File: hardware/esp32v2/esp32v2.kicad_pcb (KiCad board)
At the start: 4 copper layers, 20 x 25.5 mm, 26 parts, among them J1 Conn_01x02, J2 Conn_01x02, J3 Conn_01x10, U1 ESP32-S3, Y2 40MHz(10ppm)

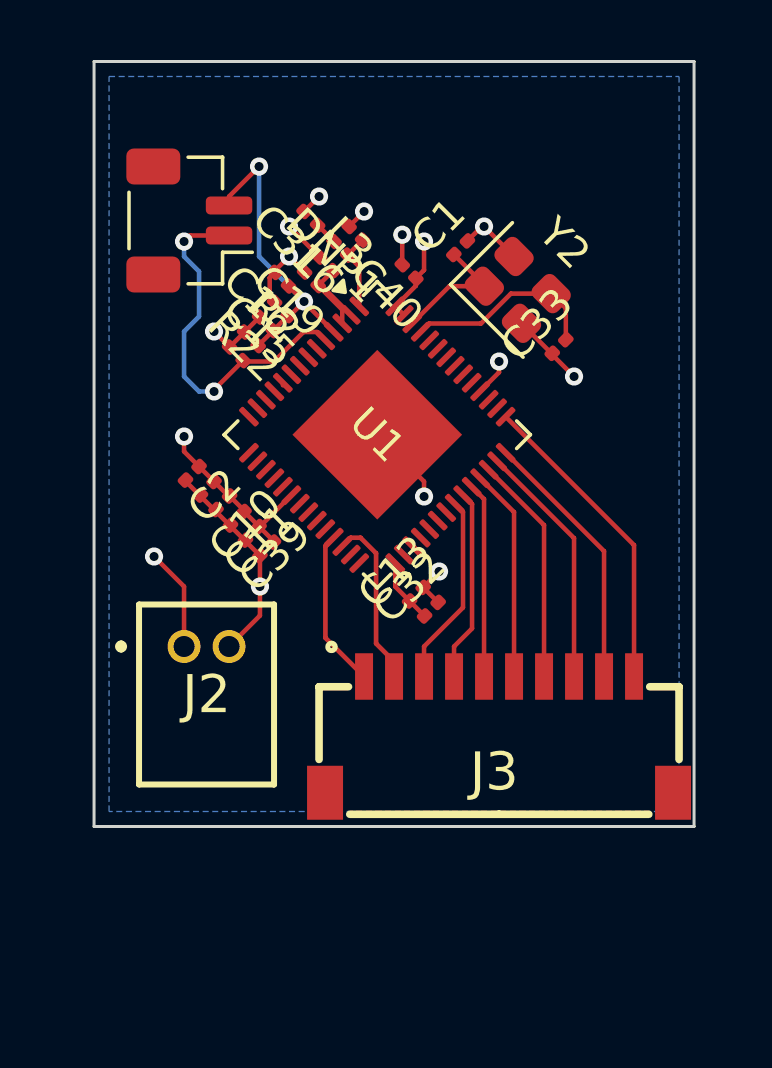
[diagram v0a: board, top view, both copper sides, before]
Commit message: wip
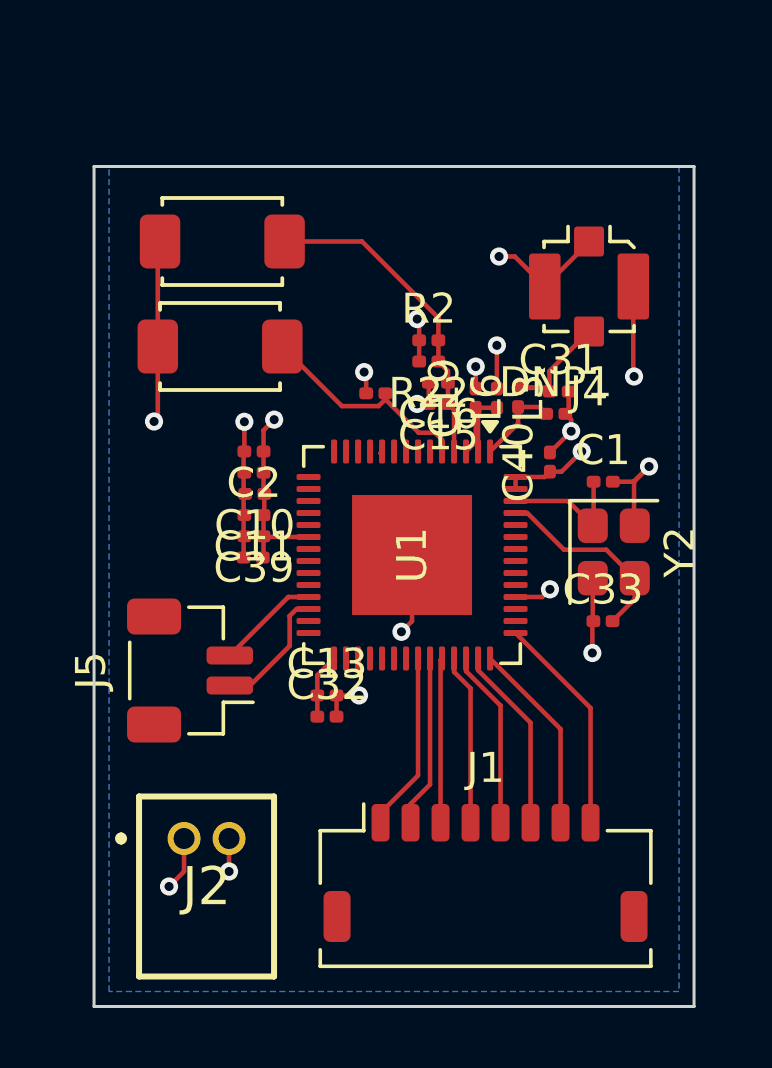
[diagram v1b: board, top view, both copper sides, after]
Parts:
- removed J3: Conn_01x10, LIB_SM10B-SRSS-TB_LF__SN_:SM10B-SRSS-TB
- added J4: Conn_01x02, Connector_Coaxial:U.FL_Molex_MCRF_73412-0110_Vertical, F.Cu at (118.5, 40.5)
- added J5: Conn_01x02, Connector_JST:JST_SH_BM02B-SRSS-TB_1x02-1MP_P1.00mm_Vertical, F.Cu at (105.2, 53.3)
- added S1: Tactile Button, 160gf, PCM_JLCPCB:SW_TS-1088-AR02016, F.Cu at (106.2, 42.5)
- added S2: Tactile Button, 160gf, PCM_JLCPCB:SW_TS-1088-AR02016, F.Cu at (106.3, 39.0)
- C31: value 15pF -> 4pF
- DNP1: value 15pF -> 5pF
- J1: value Conn_01x02 -> Conn_01x08; footprint Connector_JST:JST_SH_BM02B-SRSS-TB_1x02-1MP_P1.00mm_Vertical -> Connector_JST:JST_SHL_SM08B-SHLS-TF_1x08-1MP_P1.00mm_Horizontal
- L6: value 4.7nH -> 1.8nH
- moved J1 23.9 mm to (115.0, 60.0), turned to 0 degrees
- moved C31 10.1 mm to (117.5, 44.0), turned to 0 degrees
- moved Y2 9.30 mm to (119.3, 49.3), turned to -90 degrees
- moved C33 9.27 mm to (119.0, 51.7), turned to 0 degrees
- moved C1 9.13 mm to (119.0, 47.0), turned to 0 degrees
- moved DNP1 8.98 mm to (117.4, 44.7), turned to 0 degrees
- moved C40 7.90 mm to (117.2, 46.4), turned to 90 degrees
- moved L6 7.72 mm to (116.1, 44.2), turned to 90 degrees
- moved L3 7.24 mm to (115.4, 44.2), turned to -90 degrees
- moved C19 6.77 mm to (114.7, 44.2), turned to 90 degrees
- moved J2 6.40 mm to (105.0, 58.9)
- moved C16 6.26 mm to (113.5, 43.7), turned to 180 degrees
- moved C15 6.12 mm to (113.5, 44.4), turned to 180 degrees
- moved R2 5.91 mm to (113.2, 42.3), turned to 0 degrees
- moved R22 5.56 mm to (113.2, 43.0), turned to 180 degrees
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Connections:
- J1 pad 1: IO0 -> IO48
- J1 pad 2: EN -> IO47
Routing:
- net GND: track 20.8 -> 33.4 mm, vias 9 -> 12
- net VDD_CPU: track 25.8 -> 15.9 mm, vias 6 -> 7
- net IO0: track 12.4 -> 7.59 mm, vias 2 -> 0
- net Net-(J4-Pin_1): track 0.77 -> 4.13 mm
- net IO38: track 10.4 -> 7.36 mm
- net IO37: track 8.82 -> 6.45 mm
- net IO36: track 8.24 -> 6.20 mm
- net USB_D-: track 5.28 -> 3.43 mm
- net IO35: track 7.66 -> 5.95 mm
- net USB_D+: track 5.81 -> 4.27 mm
- net IO34: track 7.08 -> 5.70 mm
- net IO33: track 6.50 -> 5.50 mm
- net EN: track 11.1 -> 10.9 mm, vias 2 -> 0
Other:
- board size 20 x 25.5 mm -> 20 x 28 mm
